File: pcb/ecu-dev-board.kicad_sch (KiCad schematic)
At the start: 0 parts

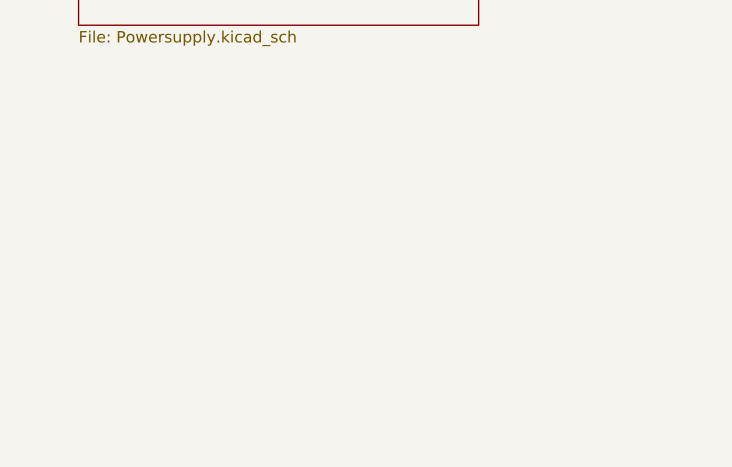
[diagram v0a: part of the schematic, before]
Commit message: added connector and simulation link
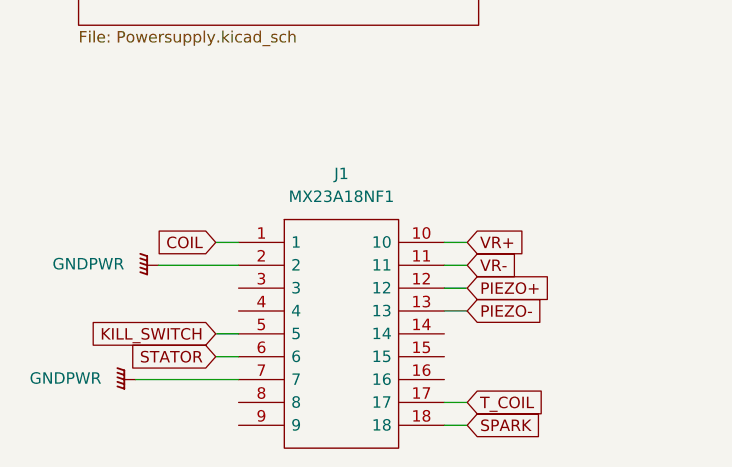
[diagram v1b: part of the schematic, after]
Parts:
- added J1: MX23A18NF1, MX23A18NF1, symbol SamacSys_Parts:MX23A18NF1
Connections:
- new net COIL: J1.1
- new net GNDPWR: J1.2, J1.7
- new net KILL_SWITCH: J1.5
- new net PIEZO+: J1.12
- new net PIEZO-: J1.13
- new net SPARK: J1.18
- new net STATOR: J1.6
- new net T_COIL: J1.17
- new net VR+: J1.10
- new net VR-: J1.11
